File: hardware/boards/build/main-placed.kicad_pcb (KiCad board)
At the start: 4 copper layers, 140 x 84 mm, 151 parts

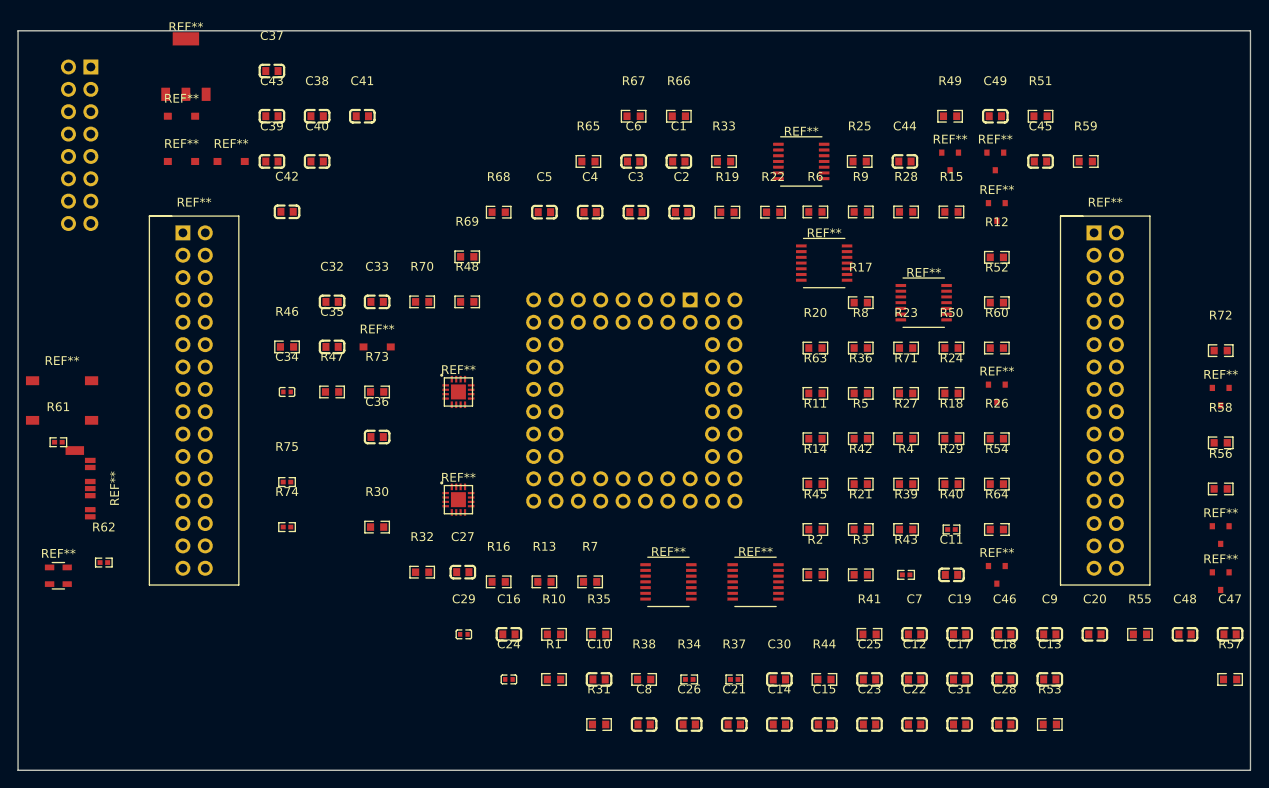
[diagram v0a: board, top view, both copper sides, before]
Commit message: Parts audit complete
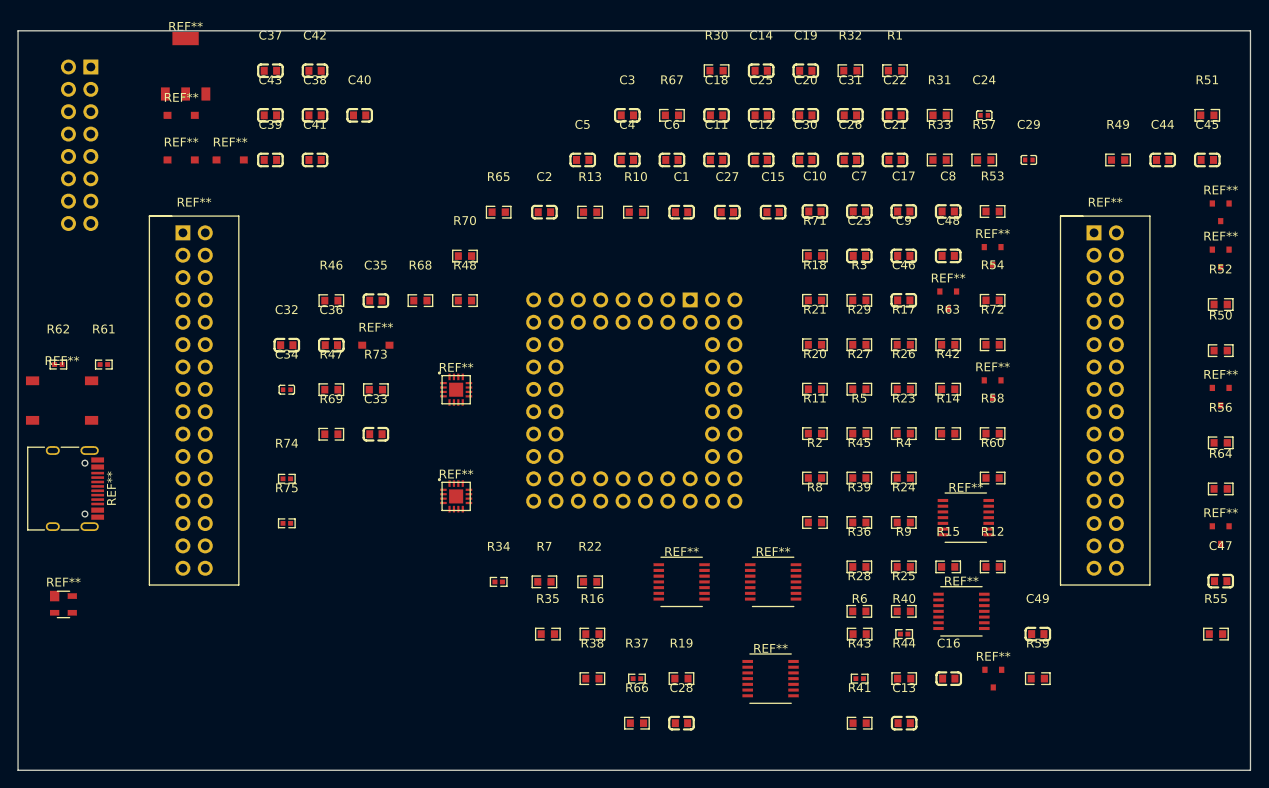
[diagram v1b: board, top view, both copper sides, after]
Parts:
- removed the REF** at (24.2, 14.8)
- removed the REF** at (40.8, 35.9)
- removed the REF** at (105.9, 14.8)
- removed the REF** at (136.6, 62.5)
- removed the REF** at (111.2, 20.6)
- removed the REF** at (111.0, 14.8)
- removed the REF** at (73.9, 62.6)
- removed the REF** at (91.6, 26.4)
- removed the REF** at (102.9, 30.9)
- removed the REF** at (50.0, 53.3)
- removed the REF** at (18.6, 14.8)
- removed the REF** at (83.8, 62.6)
- removed the REF** at (50.0, 41.0)
- removed the REF** at (111.2, 61.8)
- removed the REF** at (18.6, 9.70)
- removed the REF** at (89.0, 14.8)
- added REF**: SOT-23, BAT54S:SOT-23, F.Cu at (136.6, 25.9)
- added REF**: TSSOP-14, OPA4171AIPWR:TSSOP-14, F.Cu at (107.2, 65.9)
- added REF**: WQFN-16, DAC80508ZRTER:WQFN-16, F.Cu at (49.8, 52.9)
- added REF**: SOD-123, B5819W:SOD-123, F.Cu at (40.6, 35.7)
- added REF**: SOT-23, BAT54S:SOT-23, F.Cu at (136.6, 20.6)
- added REF**: SOD-123, B5819W:SOD-123, F.Cu at (24.1, 14.7)
- added REF**: SOT-23, BAT54S:SOT-23, F.Cu at (110.8, 73.6)
- added REF**: TSSOP-14, OPA4171AIPWR:TSSOP-14, F.Cu at (75.4, 62.6)
- added REF**: TSSOP-14, OPA4171AIPWR:TSSOP-14, F.Cu at (85.8, 62.6)
- added REF**: SOD-123, B5819W:SOD-123, F.Cu at (18.5, 14.7)
- added REF**: TSSOP-14, OPA4171AIPWR:TSSOP-14, F.Cu at (85.5, 73.6)
- added REF**: WQFN-16, DAC80508ZRTER:WQFN-16, F.Cu at (49.8, 40.8)
- added REF**: TSSOP-14, OPA4171AIPWR:TSSOP-14, F.Cu at (107.7, 55.3)
- added REF**: SOT-23, BAT54S:SOT-23, F.Cu at (105.7, 30.6)
- added REF**: SOD-123, B5819W:SOD-123, F.Cu at (18.5, 9.60)
- added REF**: SOT-23, BAT54S:SOT-23, F.Cu at (110.7, 25.6)
- moved C29 83.8 mm to (114.8, 14.7)
- moved C24 83.8 mm to (109.8, 9.60)
- moved R31 79.3 mm to (104.7, 9.60)
- moved R1 79.3 mm to (99.6, 4.53)
- moved R32 74.9 mm to (94.6, 4.53)
- moved C14 74.3 mm to (84.4, 4.53)
- moved C18 72.0 mm to (79.3, 9.60)
- moved C31 70.3 mm to (94.6, 9.60)
- moved C22 69.2 mm to (99.6, 9.60)
- moved R66 69.1 mm to (70.3, 78.6)
- moved C8 67.7 mm to (105.7, 20.5)
- moved C20 67.5 mm to (89.5, 9.60)
- moved C26 66.7 mm to (94.6, 14.7)
- moved C21 66.7 mm to (99.6, 14.7)
- moved C19 66.4 mm to (89.5, 4.53)
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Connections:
- R10 pad 1: 6 -> 9
- R11 pad 1: dac-7-2 -> dac-7-1
- R13 pad 1: 7 -> dac-10
- R16 pad 1: 8 -> 11
- R23 pad 1: dac-7 -> 7
- R37 pad 1: dac-7-1 -> dac-7
- R39 pad 1: dac-7-1 -> dac-7
- R61 pad 1: 5-1 -> 3
- R62 pad 1: 6-1 -> 11-1
- R7 pad 1: 5 -> 8
- R75 pad 2: 3 -> DP
- R9 pad 1: dac-7-2 -> dac-7-1
- REF** pad 1: VBUS -> hv
- REF** pad 2: hv -> VBUS
- REF** pad 4: DM -> DP
- REF** pad 5: 5-1 -> DM
- REF** pad 6: 6-1 -> 6
- REF** pad 7: hv -> VBUS
- REF** pad 2: c_filter-power-hv-4 -> c_vio2-power-hv
- REF** pad 3: c_vio2-power-hv -> c_filter-power-hv-3
- REF** pad 1: BASE -> hv
- REF** pad 2: hv -> BASE-1
- REF** pad 3: COLLECTOR -> COLLECTOR-1
- REF** pad 23: i2c_sda -> 23
- REF** pad 24: i2c_scl -> i2c_sda
- REF** pad 25: 25 -> i2c_scl
- REF** pad 1: BASE-1 -> hv
- REF** pad 2: hv -> BASE
- REF** pad 3: COLLECTOR-1 -> COLLECTOR
- REF** pad 3: 3 -> DP
